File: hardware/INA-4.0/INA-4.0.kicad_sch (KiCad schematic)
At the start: 20 parts, among them J1 Conn_01x05, U1 OPA365, U2 OPA365, U3 OPA365, U4 AMS1117-1.8

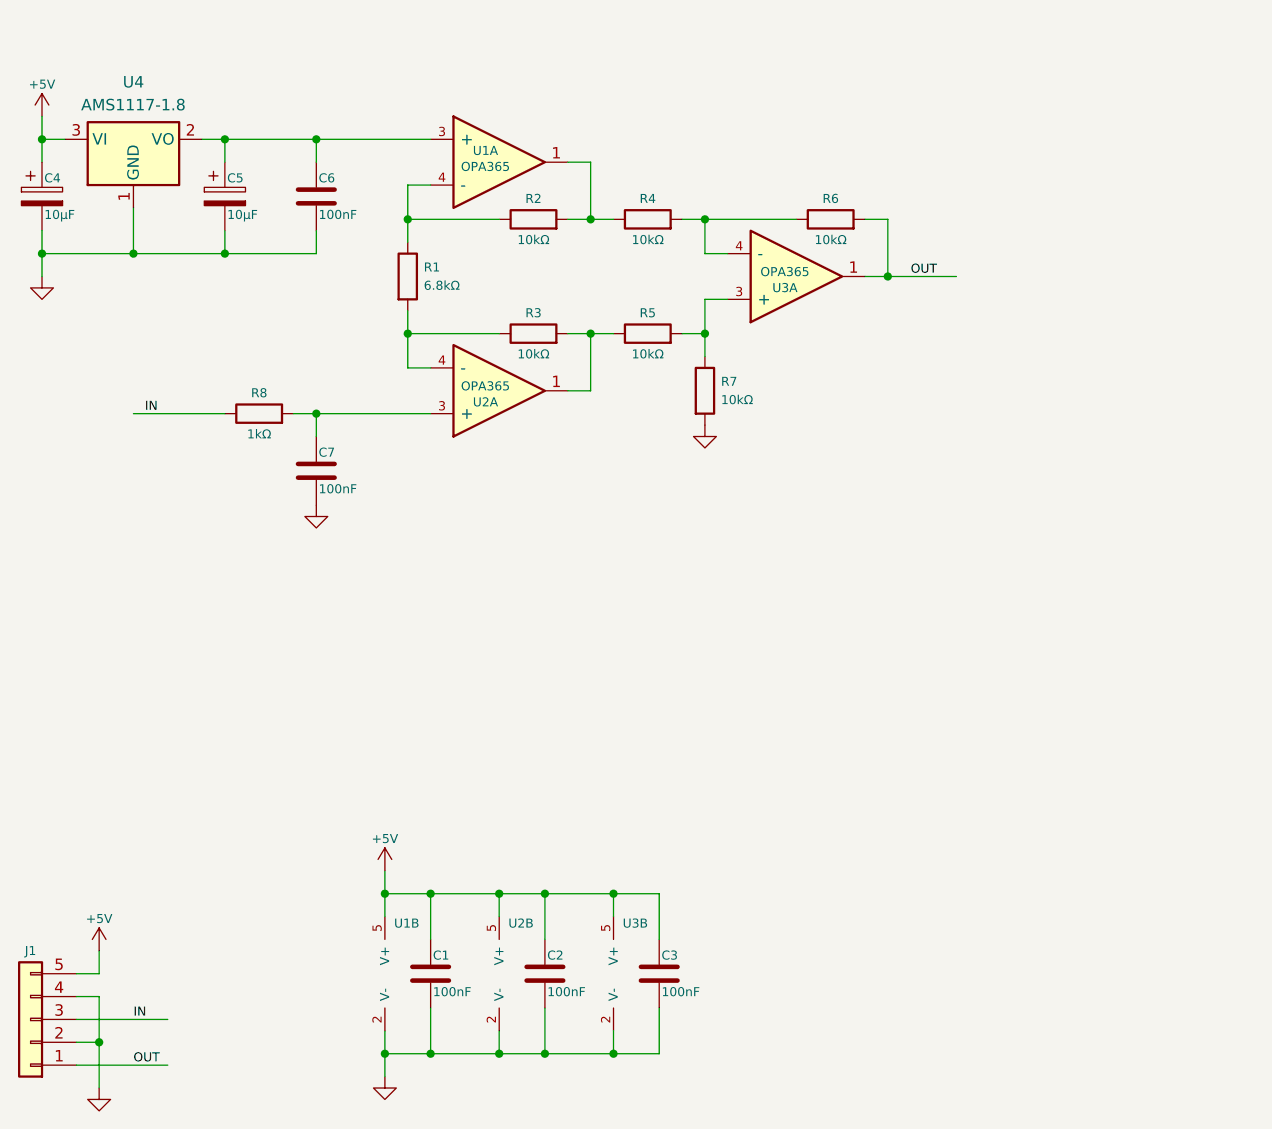
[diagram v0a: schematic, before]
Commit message: modified:   .DS_Store 	new file:   hardware/INA-3.1/INA-3-backups/INA-3-2026-04-16_161548.zip 	new file:   hardware/INA-3.1/INA-3-backups/INA-3-2026-04-16_162307.zip 	new file:   hardware/INA-3.1/INA-3-backups/INA-3-2026-04-16_163207.zip 	new file:   hardware/INA-3.1/INA-3-backups/INA-3-2026-04-17_160528.zip 	new file:   hardware/INA-3.1/INA-3-backups/INA-3-2026-04-17_161450.zip 	new file:   hardware/INA-3.1/INA-3-backups/INA-3-2026-04-17_162010.zip 	new file:   hardware/INA-3.1/INA-3-backups/INA-3-2026-04-17_162549.zip 	new file:   hardware/INA-3.1/INA-3-backups/INA-3-2026-04-17_163140.zip 	renamed:    hardware/INA-3/INA-3-backups/INA-3-2026-04-20_085258.zip -> hardware/INA-3.1/INA-3-backups/INA-3-2026-04-20_085258.zip 	new file:   hardware/INA-3.1/INA-3-backups/INA-3-2026-04-20_085822.zip 	new file:   hardware/INA-3.1/INA-3-backups/INA-3-2026-04-20_090419.zip 	new file:   hardware/INA-3.1/INA-3-backups/INA-3-2026-04-20_091140.zip 	new file:   hardware/INA-3.1/INA-3-backups/INA-3-2026-04-20_092653.zip 	new file:   hardware/INA-3.1/INA-3-backups/INA-3-2026-04-20_144439.zip 	new file:   hardware/INA-3.1/INA-3.1-backups/INA-3.1-2026-04-20_160434.zip 	new file:   hardware/INA-3.1/INA-3.1-backups/INA-3.1-2026-04-20_161047.zip 	new file:   hardware/INA-3.1/INA-3.1-backups/INA-3.1-2026-04-20_161551.zip 	new file:   hardware/INA-3.1/INA-3.1-backups/INA-3.1-2026-04-20_162147.zip 	new file:   hardware/INA-3.1/INA-3.1-backups/INA-3.1-2026-04-20_163149.zip 	new file:   hardware/INA-3.1/INA-3.1-backups/INA-3.1-2026-04-21_104126.zip 	new file:   hardware/INA-3.1/INA-3.1-backups/INA-3.1-2026-04-21_105025.zip 	new file:   hardware/INA-3.1/INA-3.1-backups/INA-3.1-2026-04-21_105750.zip 	new file:   hardware/INA-3.1/INA-3.1-backups/INA-3.1-2026-04-21_110437.zip 	new file:   hardware/INA-3.1/INA-3.1-backups/INA-3.1-2026-04-21_143841.zip 	new file:   hardware/INA-3.1/INA-3.1-backups/INA-3.1-2026-04-21_154136.zip 	renamed:    hardware/INA-3/_autosave-INA-3.kicad_pcb -> hardware/INA-3.1/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
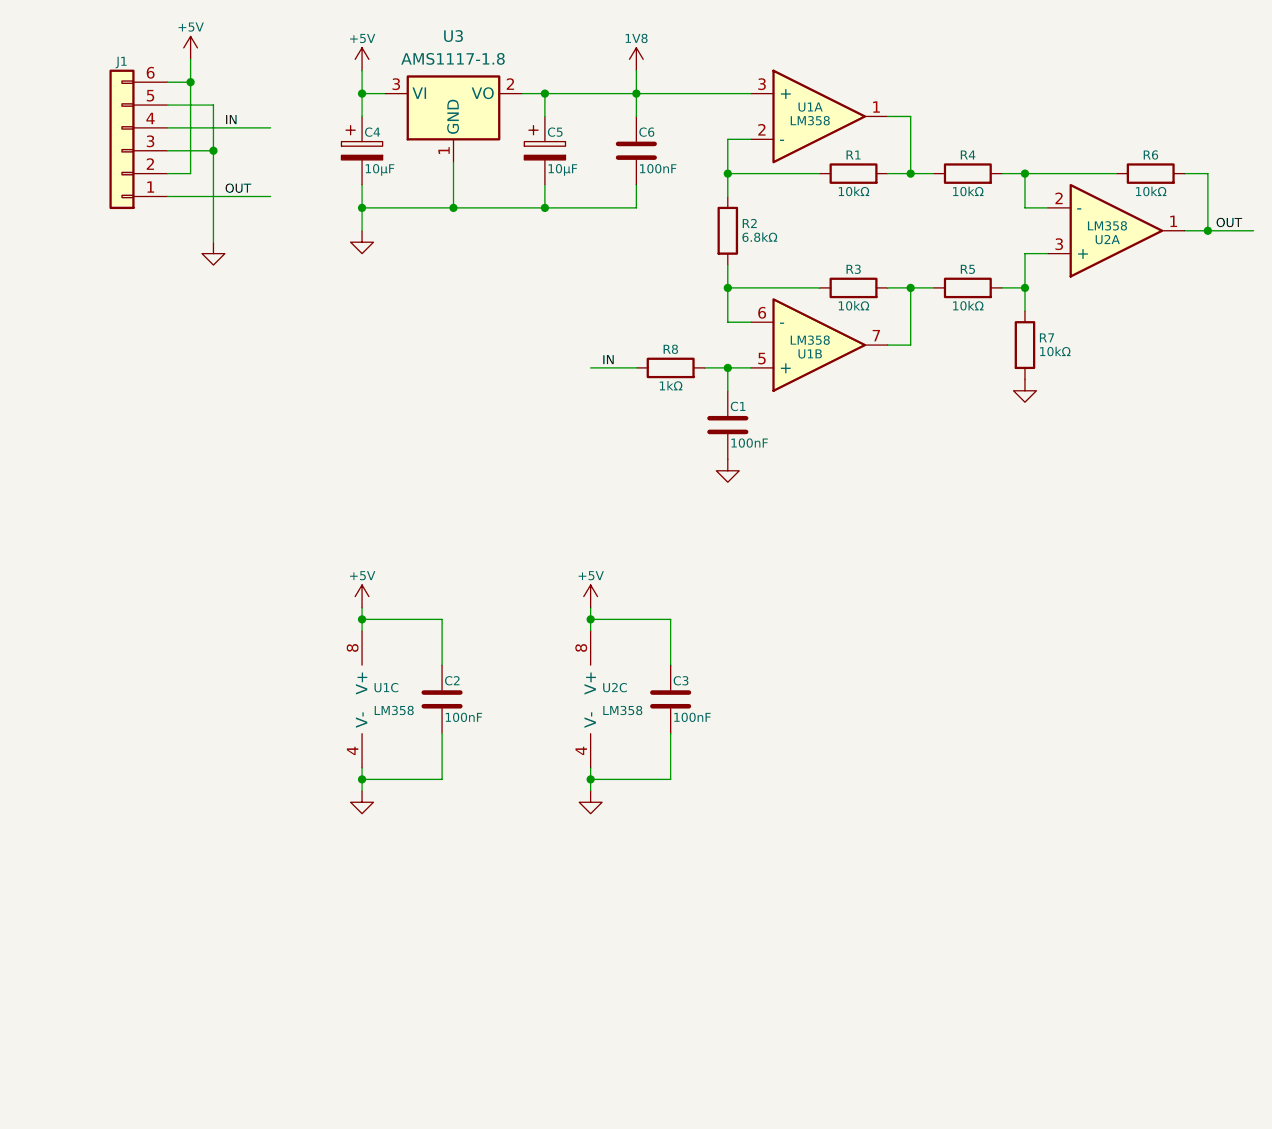
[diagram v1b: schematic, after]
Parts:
- removed C7: 100nF, Capacitor_SMD:C_0805_2012Metric_Pad1.18x1.45mm_HandSolder, symbol Device:C
- removed J1: Conn_01x05, Connector_PinHeader_2.54mm:PinHeader_1x05_P2.54mm_Horizontal_2, symbol Connector_Generic:Conn_01x05
- removed U1, U2, U3: OPA365, Package_TO_SOT_SMD:SOT-23-5_HandSoldering, symbol Amplifier_Operational:OPA365xxDBV
- removed U4: AMS1117-1.8, Package_TO_SOT_SMD:SOT-223-3_TabPin2, symbol Regulator_Linear:AMS1117-1.8
- added J1: Conn_01x05, Connector_PinHeader_2.54mm:PinHeader_1x06_P2.54mm_Horizontal, symbol Connector_Generic:Conn_01x06
- added U1, U2: LM358, Package_DIP:DIP-8_W7.62mm_Socket, symbol Amplifier_Operational:LM358
- added U3: AMS1117-1.8, Package_TO_SOT_SMD:SOT-223-3_TabPin2, symbol Regulator_Linear:AMS1117-1.8
- C1, C2, C3: footprint Capacitor_SMD:C_0805_2012Metric_Pad1.18x1.45mm_HandSolder -> Capacitor_THT:C_Rect_L7.2mm_W2.5mm_P5.00mm_FKS2_FKP2_MKS2_MKP2
- R1: value 6.8kΩ -> 10kΩ; footprint Resistor_SMD:R_0805_2012Metric_Pad1.20x1.40mm_HandSolder -> Resistor_THT:R_Axial_DIN0204_L3.6mm_D1.6mm_P5.08mm_Horizontal
- R2: value 10kΩ -> 6.8kΩ; footprint Resistor_SMD:R_0805_2012Metric_Pad1.20x1.40mm_HandSolder -> Resistor_THT:R_Axial_DIN0204_L3.6mm_D1.6mm_P5.08mm_Horizontal
- R3, R4, R5, R6, R7, R8: footprint Resistor_SMD:R_0805_2012Metric_Pad1.20x1.40mm_HandSolder -> Resistor_THT:R_Axial_DIN0204_L3.6mm_D1.6mm_P5.08mm_Horizontal
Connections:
- net +5V: now also J1.2 (Pin_2), J1.6 (Pin_6), U1.8 (V+), U2.8 (V+), U3.3 (VI); no longer C1.1
- net GND: now also J1.3 (Pin_3), J1.5 (Pin_5), U1.4 (V-), U2.4 (V-), U3.1 (GND)
- net IN: now also J1.4 (Pin_4)
- net OUT: now also J1.1 (Pin_1), U2.1
- net at R4.1: now also R1.2, U1.1; no longer R2.2
- net at R4.2, R6.1: now also U2.2 (-)
- net at R5.2, R7.1: now also U2.3 (+)
- net at R1.1, R2.1: now also U1.2 (-)
- net 1V8: now reaches C5.1, C6.1
- net 1V8: now also U1.3 (+), U3.2 (VO)
- net at R3.1: now also R2.2, U1.6 (-); no longer R1.2
- net at R3.2, R5.1: now also U1.7
- net at R8.2: now also C1.1, U1.5 (+)
